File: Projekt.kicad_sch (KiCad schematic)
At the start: 60 parts, among them Q1 CSD19505, Q4 Si2306, Q5 2N3904, Q6 2N3904, U1 ACS712, U10 ADS1015, U2 B1212S, U3 AMS1117-5.0, U4 AMS1117-3.3, U5 XL7005A, U6 XL7005A, U7 IR2104, U9 CH340G

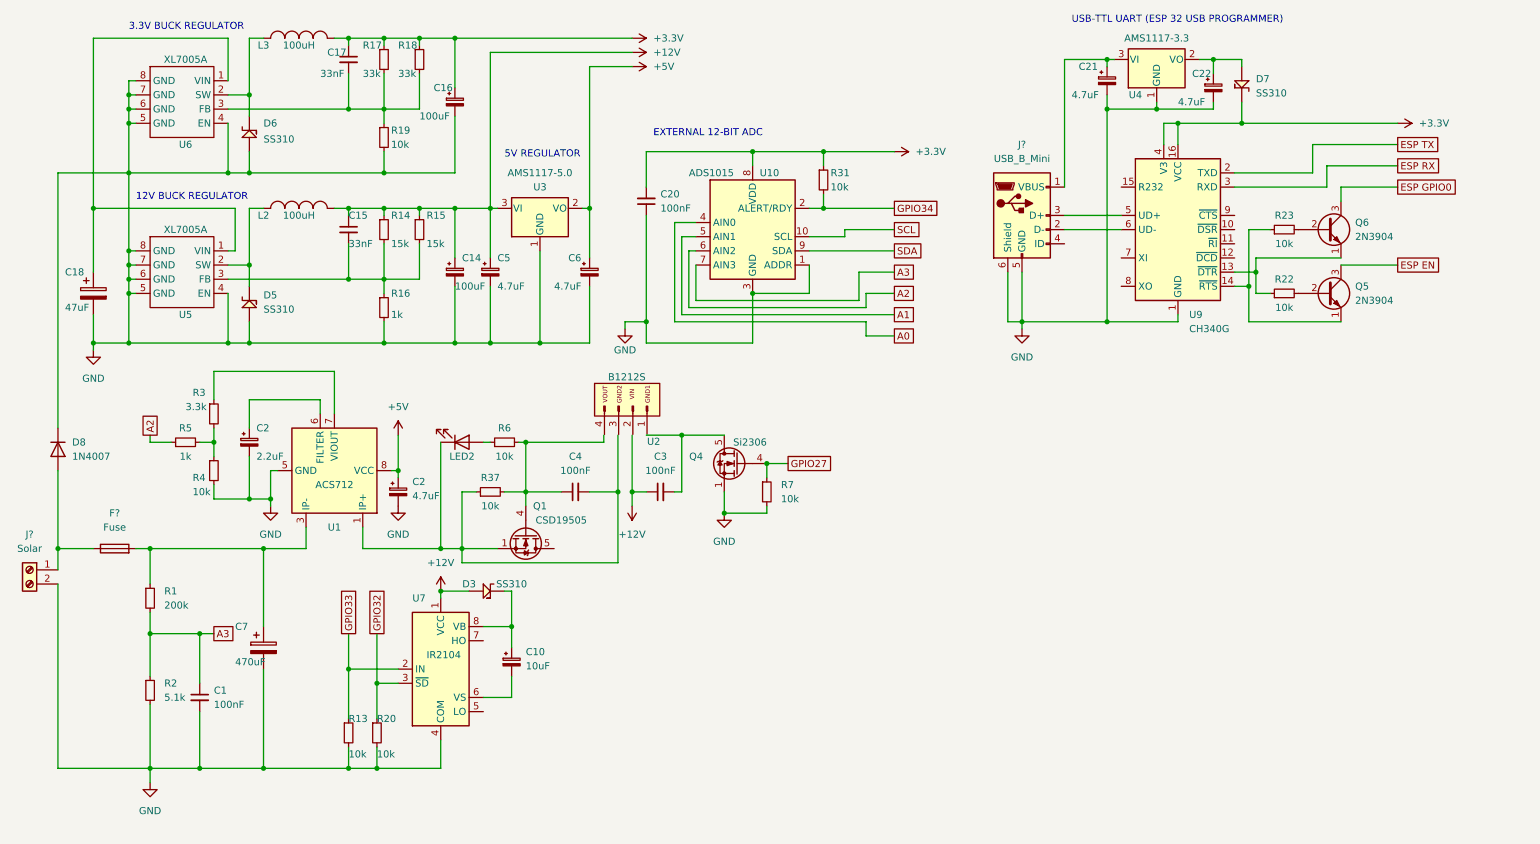
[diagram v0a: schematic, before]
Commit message: Schaltplan fertig ?
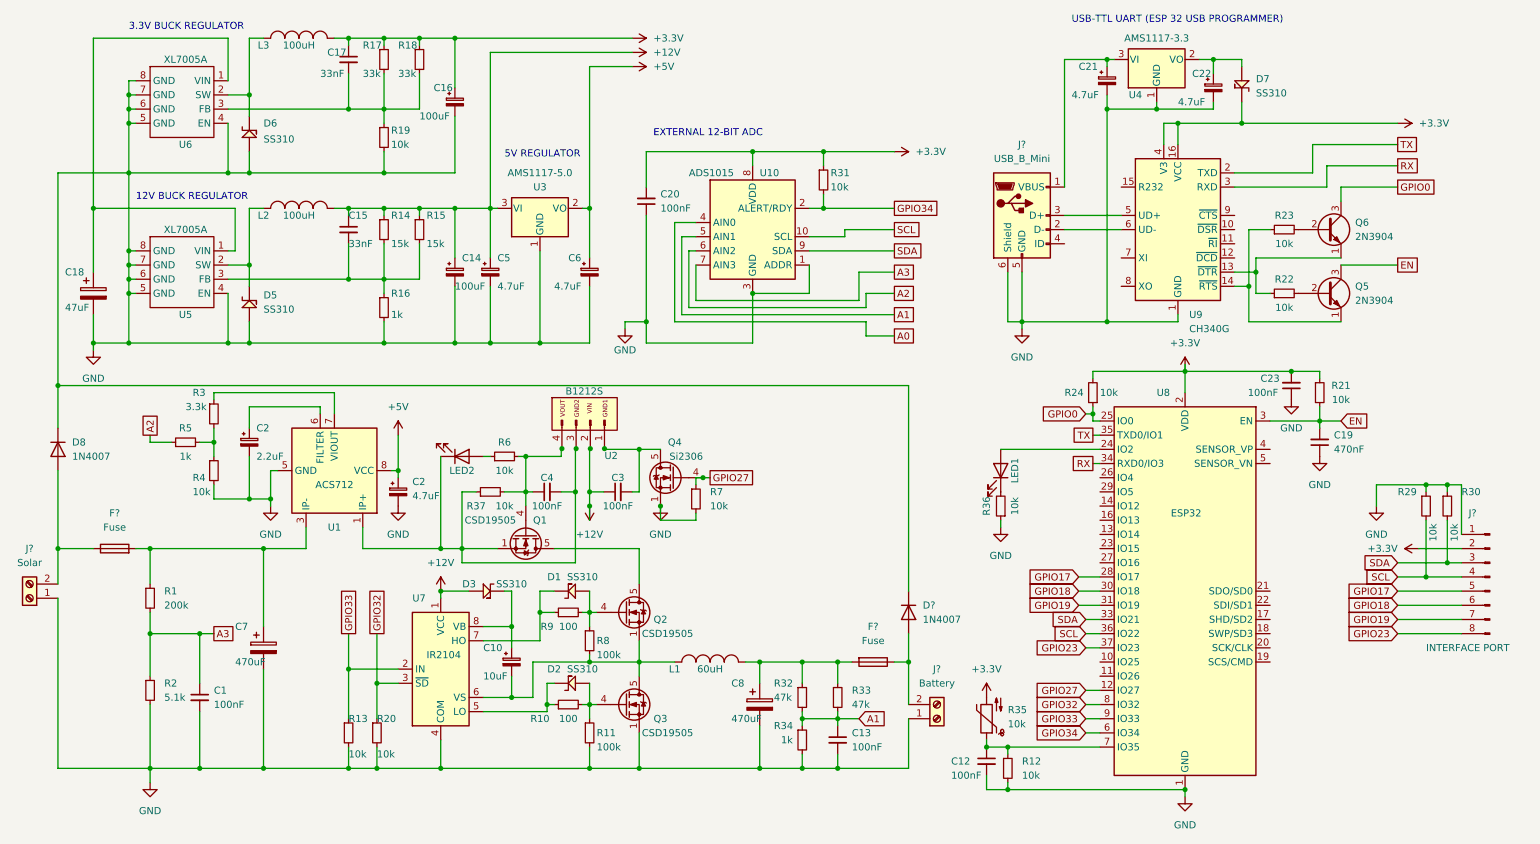
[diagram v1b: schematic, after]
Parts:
- added C12, C13, C23: 100nF, symbol Device:C_Small
- added C19: 470nF, symbol Device:C_Small
- added C8: 470uF, symbol Device:C_Polarized
- added D1, D2: SS310, Diode_SMD:D_SMB, symbol footprint:SS310
- added D?: 1N4007, Diode_THT:D_DO-41_SOD81_P10.16mm_Horizontal, symbol Diode:1N4007
- added F?: Fuse, symbol Device:Fuse
- added J?: INTERFACE PORT, symbol Connector:Conn_01x08_Male
- added J?: Battery, symbol Connector:Screw_Terminal_01x02
- added L1: 60uH, Inductor_THT:L_Toroid_Vertical_L21.6mm_W11.4mm_P7.62mm_Pulse_KM-3, symbol footprint:SMD_INDUCTOR_CD54
- added LED1: LED, symbol Device:LED
- added Q2, Q3: CSD19505, Package_TO_SOT_THT:TO-220-3_Vertical, symbol Transistor_FET:CSD19502Q5B
- added R10, R9: 100, symbol Device:R_Small
- added R11, R8: 100k, symbol Device:R_Small
- added R12, R21, R24, R29, R30, R36: 10k, symbol Device:R_Small
- added R32, R33: 47k, symbol Device:R_Small
- added R34: 1k, symbol Device:R_Small
- added R35: 10k, symbol Device:Thermistor_NTC
- added U8: ESP32, RF_Module:ESP32-WROOM-32, symbol RF_Module:ESP32-WROOM-32
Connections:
- net +3.3V: now also C23.2, J?.2 (Pin_2), R21.1, R24.2, R35.2, U8.2 (VDD)
- net A1: now also C13.1, R32.2, R33.2, R34.1
- net GND: now also J?.1 (Pin_1), C12.2, C13.2, C19.1, C23.1, C8.2, D?.1 (K), J?.1 (Pin_1), J?.1 (Pin_1), Q3.1 (S), Q3.2 (S), Q3.3 (S), R11.2, R12.2, R29.1, R30.1, R34.2, R36.1, U8.1 (GND), U8.15 (GND), U8.38 (GND), U8.39 (GND); no longer J?.2 (Pin_2)
- net GPIO27: now also U8.12 (IO27)
- net GPIO32: now also U8.8 (IO32)
- net GPIO33: now also U8.9 (IO33)
- net GPIO34: now also U8.6 (IO34)
- net SCL: now also J?.4 (Pin_4), R29.2, U8.36 (IO22)
- net SDA: now also J?.3 (Pin_3), R30.2, U8.33 (IO21)
- net at U7.5 (LO): now also D2.A1 (Anode), R10.1
- net at C10.2, U7.6 (VS): now also L1.1, Q2.1 (S), Q2.2 (S), Q2.3 (S), Q3.5 (D), R8.2
- net at U7.7 (HO): now also D1.A1 (Anode), R9.1
- net at Q1.5 (D): now also Q2.5 (D)
- net at D8.2 (A), F?.1: now also J?.2 (Pin_2); no longer J?.1 (Pin_1)
- net ESP EN renamed EN
- net EN: now also C19.2, R21.2, U8.3 (EN)
- net ESP GPIO0 renamed GPIO0
- net GPIO0: now also R24.1, U8.25 (IO0)
- net ESP RX renamed RX
- net RX: now also U8.34 (RXD0/IO3)
- net ESP TX renamed TX
- net TX: now also U8.35 (TXD0/IO1)
- new net: C8.1, F?.2, L1.2, R32.1, R33.1
- new net: D2.A2 (Katode), Q3.4 (G), R10.2, R11.1
- new net: C12.1, R12.1, R35.1, U8.7 (IO35)
- new net: D1.A2 (Katode), Q2.4 (G), R8.1, R9.2
- new net: D?.2 (A), F?.1, J?.2 (Pin_2)
- new net: LED1.1 (K), R36.2
- new net: LED1.2 (A), U8.24 (IO2)
- new net GPIO17: J?.5 (Pin_5), U8.28 (IO17)
- new net GPIO18: J?.6 (Pin_6), U8.30 (IO18)
- new net GPIO19: J?.7 (Pin_7), U8.31 (IO19)
- new net GPIO23: J?.8 (Pin_8), U8.37 (IO23)
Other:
- moved on the sheet: C3, C4, J?, LED2, Q4, R6, R7, U2

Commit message: Layouten...
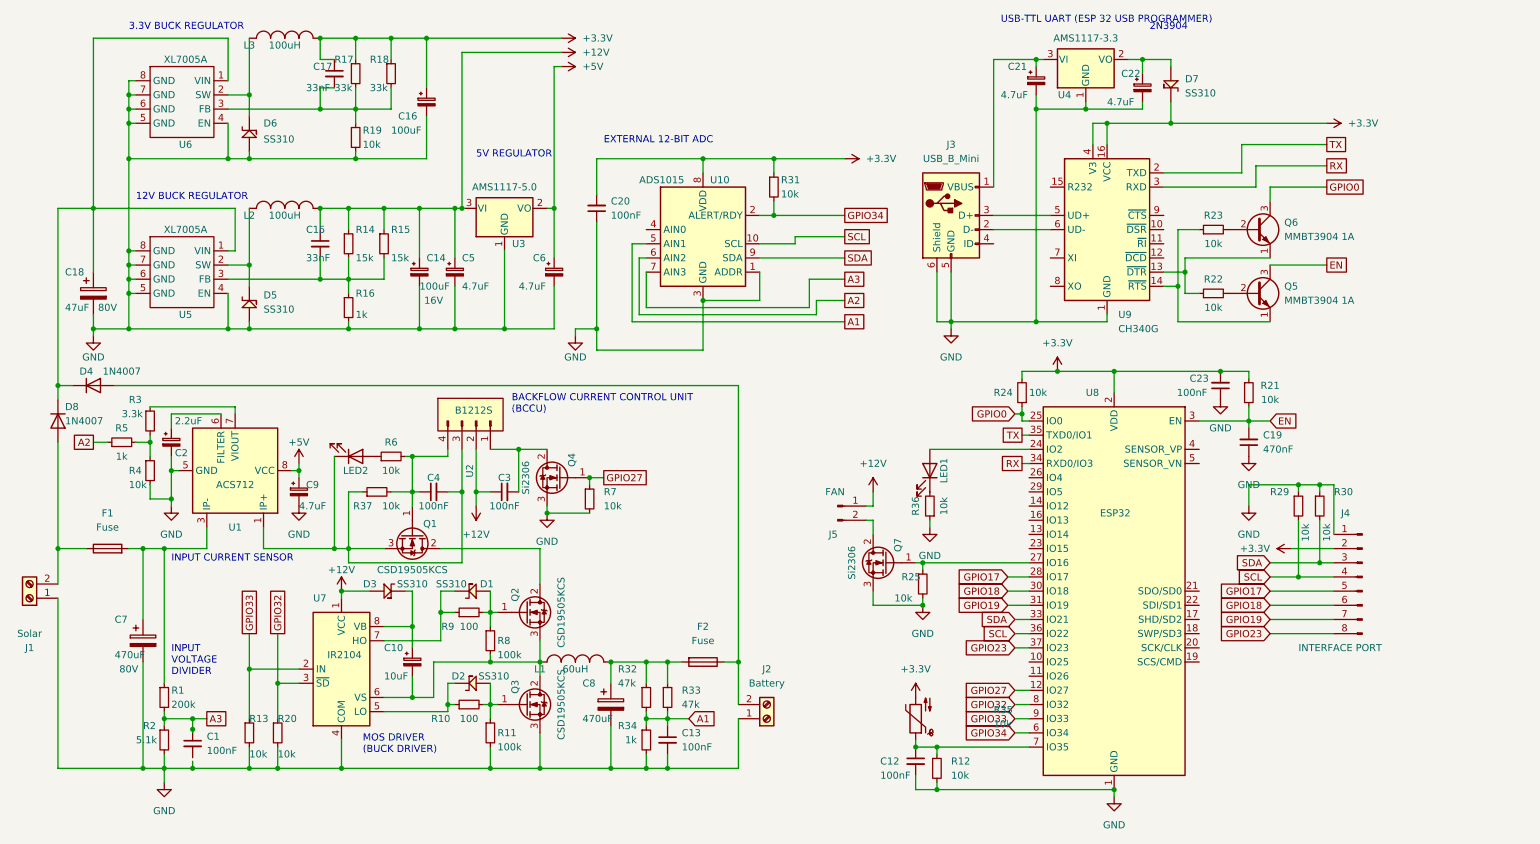
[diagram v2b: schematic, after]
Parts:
- removed Q1, Q2, Q3: CSD19505, Package_TO_SOT_THT:TO-220-3_Vertical, symbol Transistor_FET:CSD19502Q5B
- removed Q4: Si2306, Package_TO_SOT_SMD:SOT-23, symbol Transistor_FET:CSD19502Q5B
- added J5: FAN, Connector_PinHeader_2.54mm:PinHeader_1x02_P2.54mm_Vertical, symbol Connector:Conn_01x02_Male
- added Q1, Q2, Q3: CSD19505KCS, Package_TO_SOT_THT:TO-220-3_Vertical, symbol footprint:CSD19505KCS
- added Q4, Q7: Si2306, Package_TO_SOT_SMD:SOT-23, symbol footprint:CSD19505KCS
- added R25: 10k, Resistor_SMD:R_0805_2012Metric, symbol Device:R_Small
- C1, C12, C13, C15, C17, C19, C2, C20, C23, C3, C4: footprint (none) -> Capacitor_SMD:C_0603_1608Metric
- C10: footprint (none) -> Capacitor_SMD:C_Elec_5x5.4
- C14: footprint (none) -> Capacitor_SMD:C_Elec_6.3x5.8; Voltage (none) -> 16V
- C16: footprint (none) -> Capacitor_SMD:C_Elec_6.3x5.8
- C18: footprint (none) -> Capacitor_SMD:C_Elec_6.3x5.8; Voltage (none) -> 80V
- C21, C22, C5, C6: footprint (none) -> Capacitor_SMD:C_0805_2012Metric
- C7: footprint (none) -> Capacitor_THT:C_Radial_D12.5mm_H20.0mm_P5.00mm; Voltage (none) -> 80V
- C8: footprint (none) -> Capacitor_THT:C_Radial_D12.5mm_H20.0mm_P5.00mm
- C9: renamed from C2; footprint (none) -> Capacitor_SMD:C_0805_2012Metric
- D4: renamed from D?; footprint Diode_THT:D_DO-41_SOD81_P10.16mm_Horizontal -> Diode_SMD:D_SMC
- D8: footprint Diode_THT:D_DO-41_SOD81_P10.16mm_Horizontal -> Diode_SMD:D_SMC
- F1, F2: renamed from F?; footprint (none) -> Fuse:Fuse_Blade_ATO_directSolder
- J1, J2: renamed from J?; footprint (none) -> TerminalBlock_WAGO:TerminalBlock_WAGO_236-602_1x02_P10.00mm_45Degree
- J3: renamed from J?; footprint (none) -> Connector_USB:USB_Mini-B_Lumberg_2486_01_Horizontal
- J4: renamed from J?; footprint (none) -> Connector_PinHeader_2.54mm:PinHeader_1x08_P2.54mm_Vertical
- LED1, LED2: footprint (none) -> LED_SMD:LED_0805_2012Metric
- Q5, Q6: value 2N3904 -> MMBT3904 1A; footprint Package_TO_SOT_THT:TO-92_Inline -> Package_TO_SOT_SMD:SOT-23
- R1, R10, R11, R12, R13, R14, R15, R16, R17, R18, R19, R2, R20, R21, R22, R23, R24, R29, R3, R30, R31, R32, R33, R34, R35, R36, R37, R4, R5, R6, R7, R8, R9: footprint (none) -> Resistor_SMD:R_0805_2012Metric
- U2: footprint 1x04_P2.50mm -> Connector_PinHeader_2.54mm:PinHeader_1x04_P2.54mm_Vertical
- U7: footprint (none) -> Package_SO:SOIC-8_3.9x4.9mm_P1.27mm
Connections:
- net +12V: now also D3.1 (Katode), U2.2 (VIN), J5.1 (Pin_1); no longer D3.A2 (Katode)
- net +3.3V: now also D7.2 (Anode); no longer D7.A1 (Anode)
- net GND: now also D5.1 (Katode), D6.1 (Katode), Q3.3 (S), Q4.3 (S), Q7.3 (S), R25.2; no longer C1.2, D4.1 (K), D5.A2 (Katode), D6.A2 (Katode), D8.1 (K)
- net GPIO27: now also Q4.1 (G)
- net at C18.1, U5.1 (VIN), U6.1 (VIN): now also D4.1 (K), D8.1 (K)
- net at L2.1, U5.2 (SW): now also D5.2 (Anode); no longer D5.A1 (Anode)
- net at R10.1, U7.5 (LO): now also D2.2 (Anode); no longer D2.A1 (Anode)
- net at R10.2, R11.1: now also D2.1 (Katode), Q3.1 (G); no longer D2.A2 (Katode)
- net at C22.1, U4.2 (VO): now also D7.1 (Katode); no longer D7.A2 (Katode)
- net at C4.1, R37.2, R6.2: now also U2.4 (VOUT), Q1.1 (G)
- net at C4.2, LED2.1 (K), R37.1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: now also U2.3 (GND2), Q1.3 (S)
- net at C10.2, L1.1, R8.2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: now also Q2.3 (S), Q3.2 (D)
- net at R9.1, U7.7 (HO): now also D1.2 (Anode); no longer D1.A1 (Anode)
- net at C10.1, U7.8 (VB): now also D3.2 (Anode); no longer D3.A1 (Anode)
- net at C3.2: now also U2.1 (GND), Q4.2 (D)
- net at R8.1, R9.2: now also D1.1 (Katode), Q2.1 (G); no longer D1.A2 (Katode)
- net at L3.1, U6.2 (SW): now also D6.2 (Anode); no longer D6.A1 (Anode)
- net at U8.27 (IO16): now also Q7.1 (G), R25.1
- net A0: no longer names the net of U10.4 (AIN0)
- new net: J5.2 (Pin_2), Q7.2 (D)
- new net: Q1.2 (D), Q2.2 (D)
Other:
- note added: "2N3904"
- note added: "BACKFLOW CURRENT CONTROL UNIT (BCCU)"
- note added: "INPUT CURRENT SENSOR"
- note added: "INPUT VOLTAGE DIVIDER"
- note added: "MOS DRIVER (BUCK DRIVER)"
- moved on the sheet: C1, C10, C12, C13, C14, C15, C16, C17, C19, C2, C20, C21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

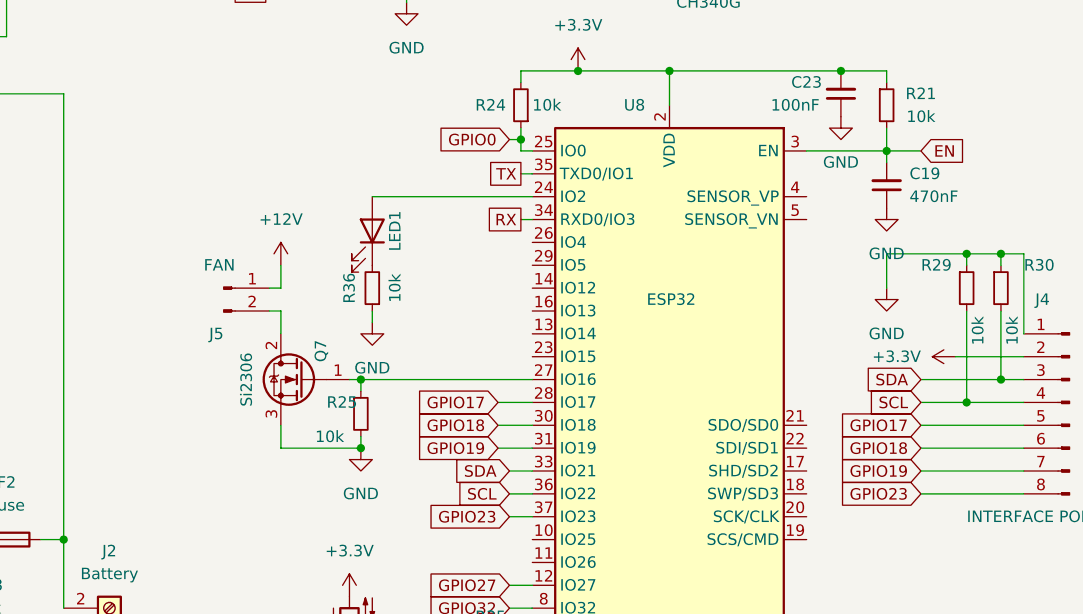
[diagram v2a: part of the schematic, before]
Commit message: So gut wie fertig ... ?
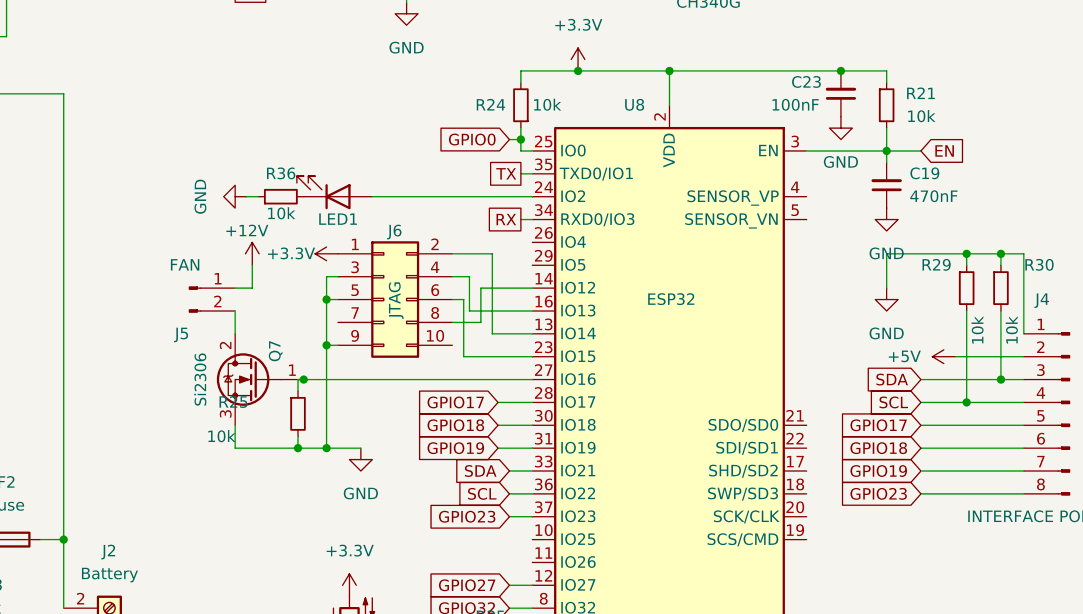
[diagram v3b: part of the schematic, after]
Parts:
- added J6: JTAG, Connector_PinHeader_1.27mm:PinHeader_2x05_P1.27mm_Vertical_SMD, symbol Connector_Generic:Conn_02x05_Odd_Even
- D4, D8: footprint Diode_SMD:D_SMC -> Diode_SMD:D_SMB
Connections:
- net +3.3V: now also J6.1 (Pin_1); no longer J4.2 (Pin_2)
- net +5V: now also J4.2 (Pin_2)
- net GND: now also J6.3 (Pin_3), J6.5 (Pin_5), J6.9 (Pin_9)
- net at U8.13 (IO14): now also J6.2 (Pin_2)
- net at U8.14 (IO12): now also J6.8 (Pin_8)
- net at U8.16 (IO13): now also J6.4 (Pin_4)
- net at U8.23 (IO15): now also J6.6 (Pin_6)
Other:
- moved on the sheet: J5, LED1, Q7, R25, R36
